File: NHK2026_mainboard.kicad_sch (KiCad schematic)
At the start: 14 parts, among them J1 ABS_Encoder, J2 SPI, J3 I2C, J4 SOLENOID_1, J5 ADC, J6 PicoScan, SW1 SW_Push, U1 TXRX_pokayoke, U2 BNO055, U3 NUCLEO-H753ZI

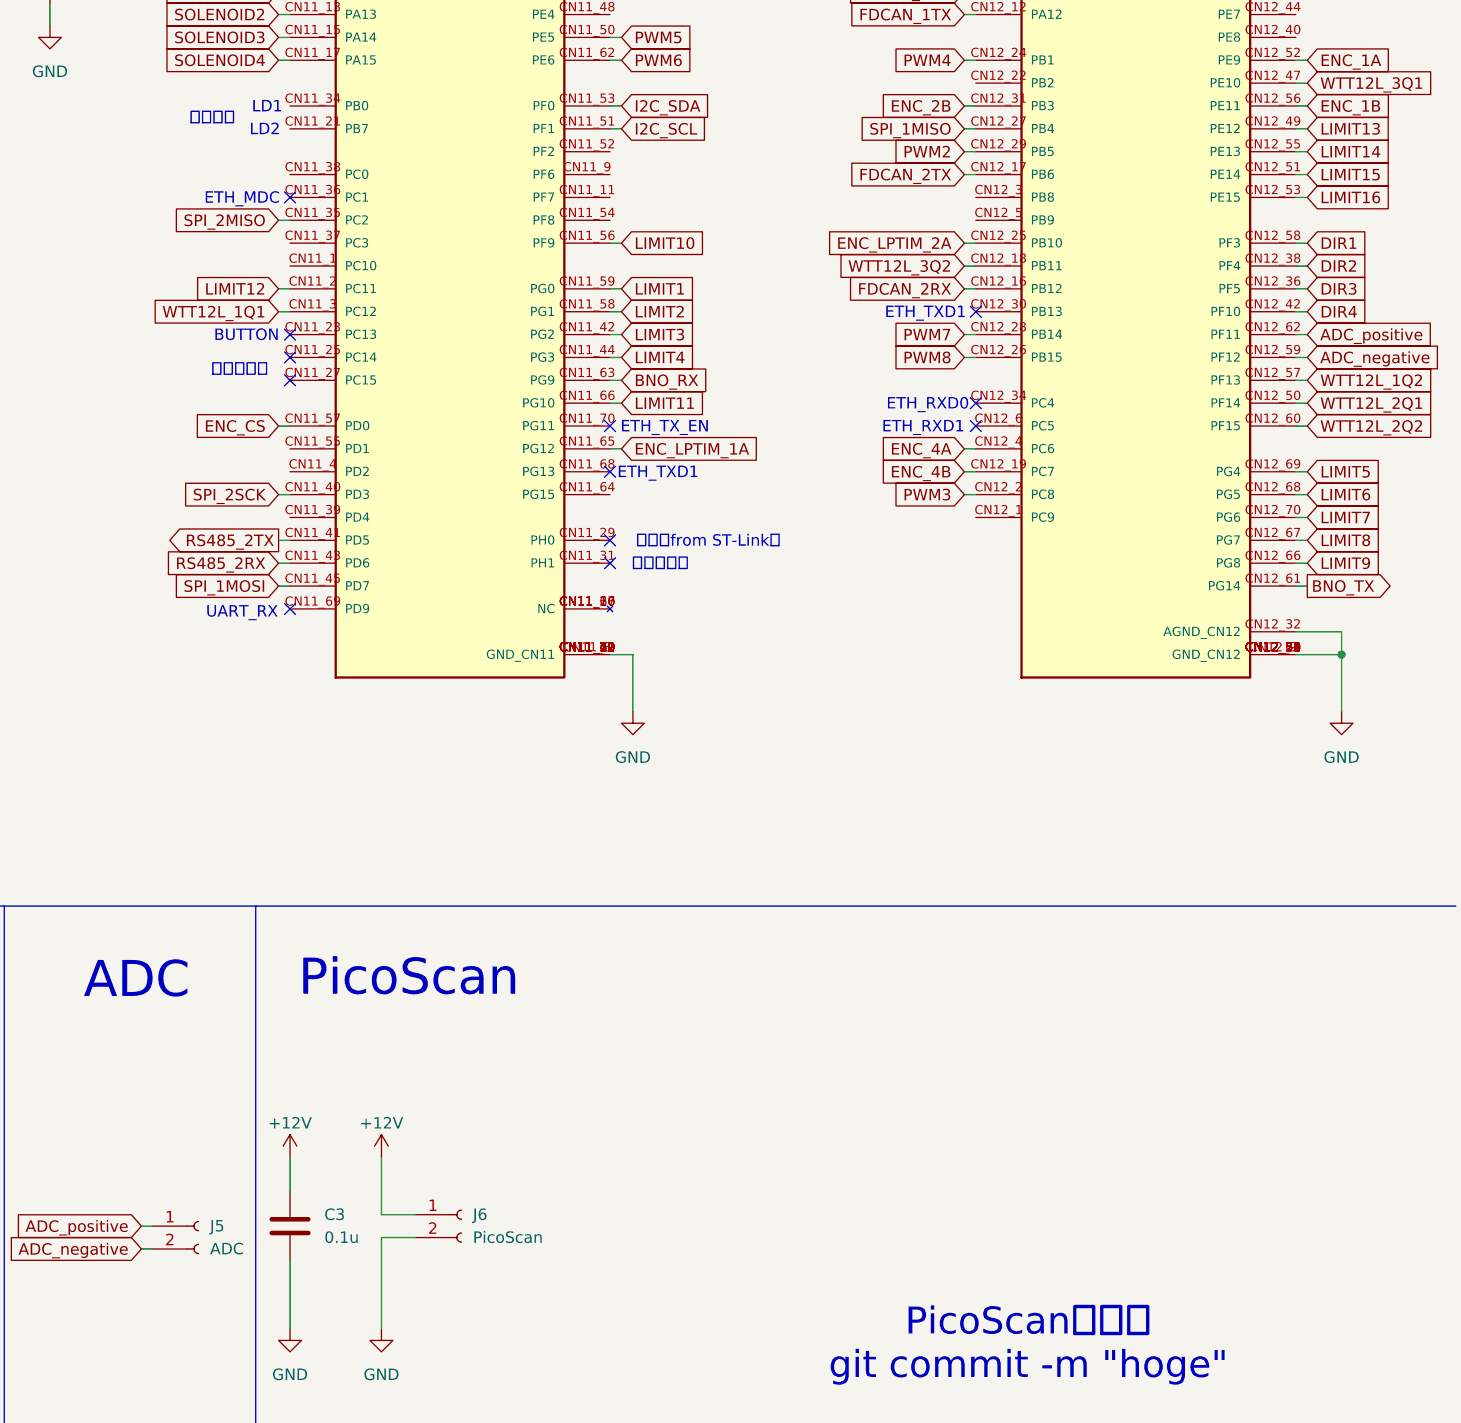
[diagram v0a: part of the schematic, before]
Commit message: メイン基板完成
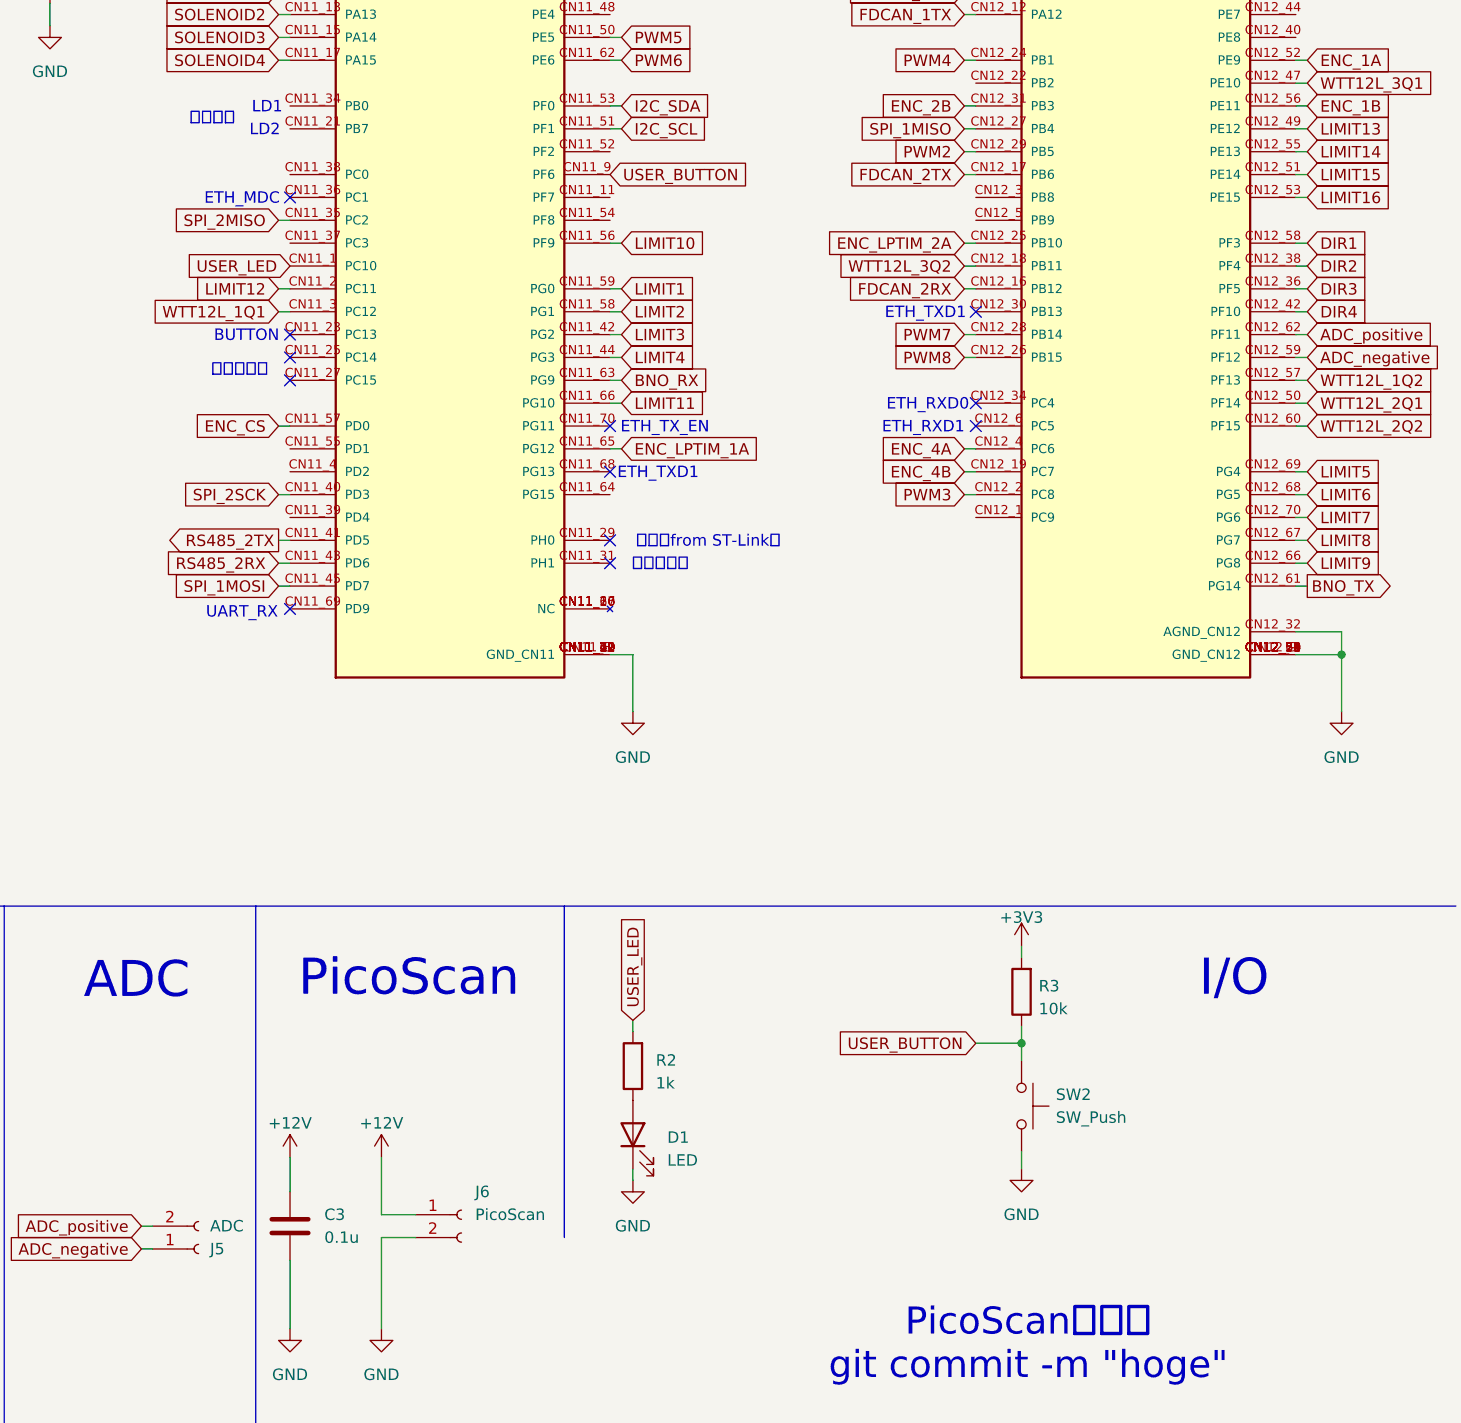
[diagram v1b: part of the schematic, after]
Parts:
- added D1: LED, LED_SMD:LED_0603_1608Metric_Pad1.05x0.95mm_HandSolder, symbol Device:LED
- added R2: 1k, Resistor_SMD:R_0603_1608Metric_Pad0.98x0.95mm_HandSolder, symbol Device:R
- added R3: 10k, Resistor_SMD:R_0603_1608Metric_Pad0.98x0.95mm_HandSolder, symbol Device:R
- added SW2: SW_Push, Button_Switch_THT:SW_PUSH_6mm, symbol Switch:SW_Push
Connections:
- net +3V3: now also R3.2
- net ADC_negative: now also J5.1 (Pin_1); no longer J5.2 (Pin_2)
- net ADC_positive: now also J5.2 (Pin_2); no longer J5.1 (Pin_1)
- net GND: now also D1.1 (K), SW2.2
- net USER_LED: now reaches U3.CN11_1 (PC10)
- net USER_LED: now also R2.2
- net USER_BUTTON: now reaches U3.CN11_9 (PF6)
- net USER_BUTTON: now also R3.1, SW2.1
- new net: D1.2 (A), R2.1
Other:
- note added: "I/O"
